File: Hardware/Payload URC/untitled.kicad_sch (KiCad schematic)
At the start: 12 parts, among them Q1 AO3400A, Q2 AO3400A

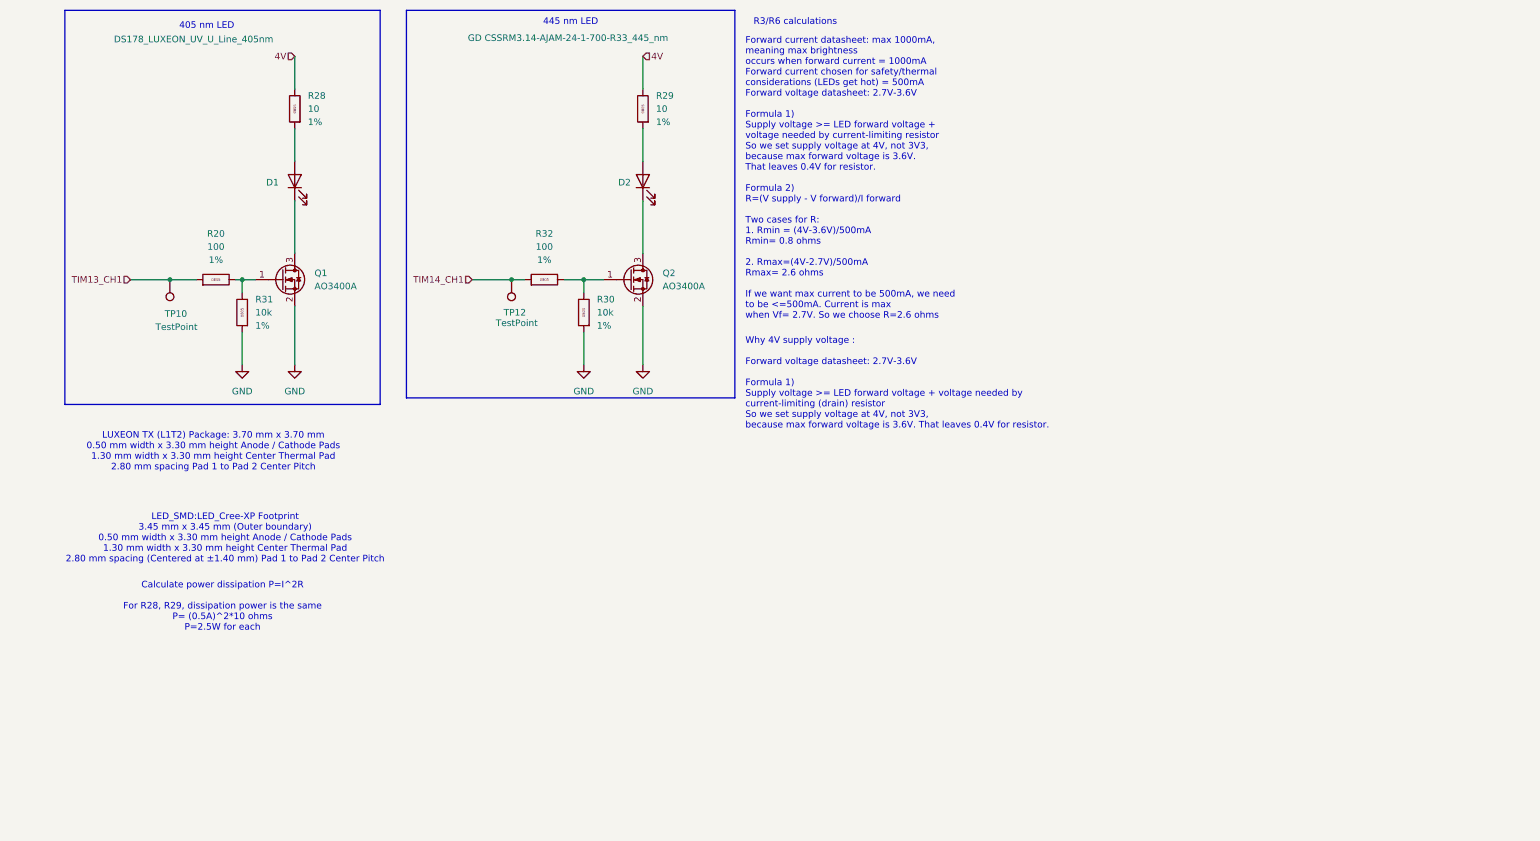
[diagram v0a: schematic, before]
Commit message: Updated files
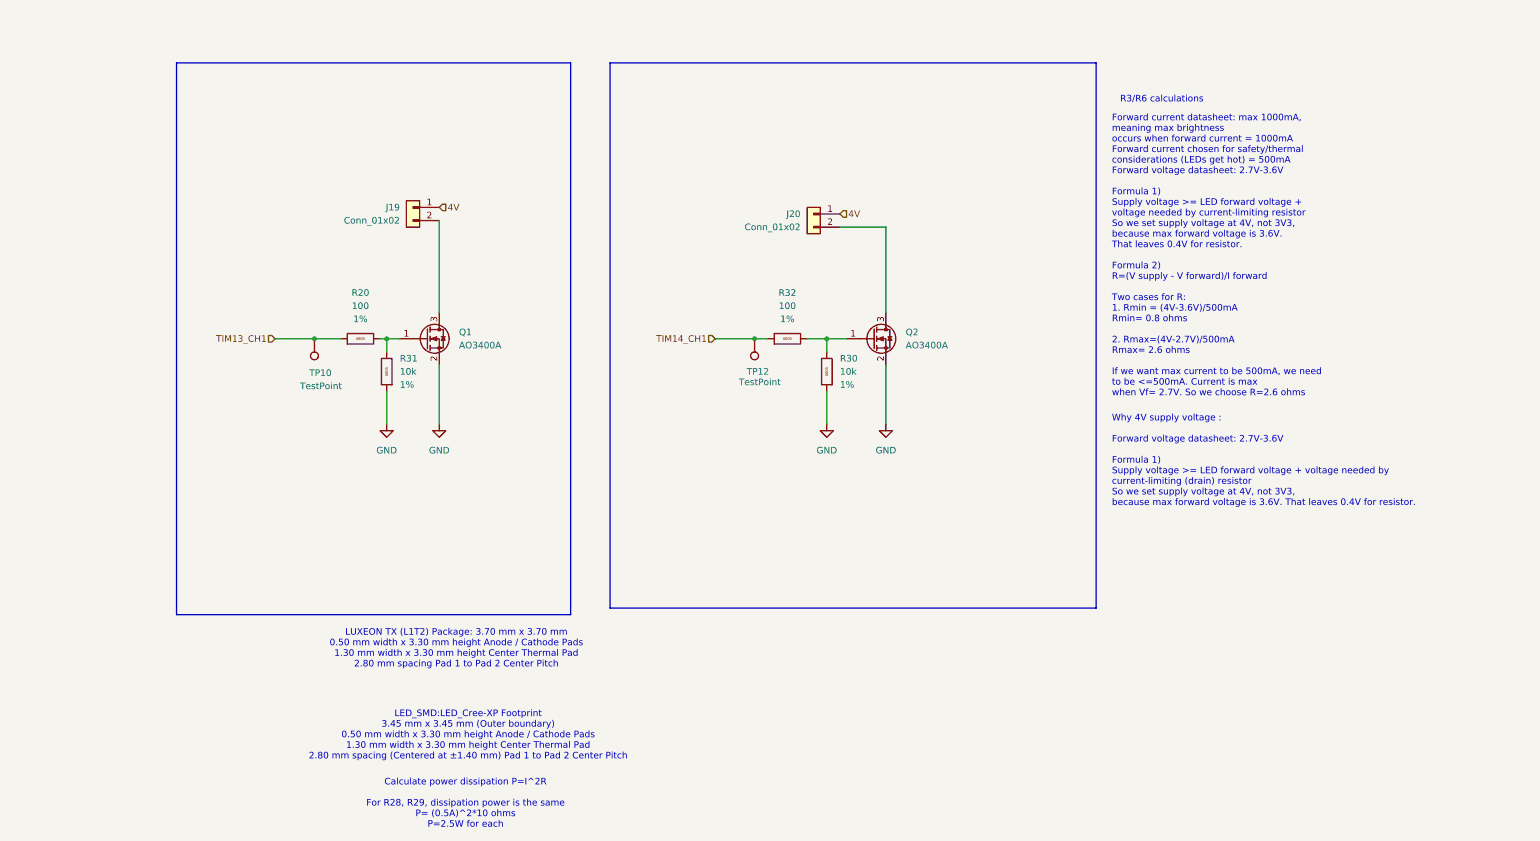
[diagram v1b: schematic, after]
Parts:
- removed D1: DS178_LUXEON_UV_U_Line_405nm, LED_SMD:LED_Cree-XP, symbol Device:LED
- removed D2: GD CSSRM3.14-AJAM-24-1-700-R33_445_nm, LED_SMD:LED_Cree-XP, symbol Device:LED
- removed R28, R29: 10, SCRB_STD_Passives:R0805, symbol SCRB_STD_Passives:R0805
- added J19, J20: Conn_01x02, SCRB_Connectors:JST-GH-SM04B-GHS-TB, symbol Connector_Generic:Conn_01x02
- TP10, TP12: footprint TestPoint:TestPoint_Pad_D2.0mm -> TestPoint:TestPoint_Loop_D2.60mm_Drill1.6mm_Beaded
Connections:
- net 4V: now also J19.1 (Pin_1), J20.1 (Pin_1)
- net at Q2.3 (D): now also J20.2 (Pin_2)
- net at Q1.3 (D): now also J19.2 (Pin_2)
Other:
- note removed: "405 nm LED"
- note removed: "445 nm LED"
- moved on the sheet: Q1, Q2, R20, R30, R31, R32, TP10, TP12

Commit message: Update
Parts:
- Q1, Q2: KiLib_Generator (none) -> package/gullwing
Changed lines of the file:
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@@
+			)
+		)
+		(property "KiLib_Generator" "package/gullwing"
+			(at 170.18 77.47 0)
+			(hide yes)
+			(show_name no)
+			(do_not_autoplace no)
+			(effects
+				(font
+					(size 1.27 1.27)
+				)
 			)
 		)
@@
 			(at 83.82 77.47 0)
 			(hide yes)
+			(show_name no)
+			(do_not_autoplace no)
+			(effects
+				(font
+					(size 1.27 1.27)
+				)
+			)
+		)
+		(property "KiLib_Generator" "package/gullwing"
+			(at 83.82 77.47 0)
+			(hide yes)
